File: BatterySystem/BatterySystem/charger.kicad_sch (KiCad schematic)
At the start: 1 part, among them U2 BQ25895RTW

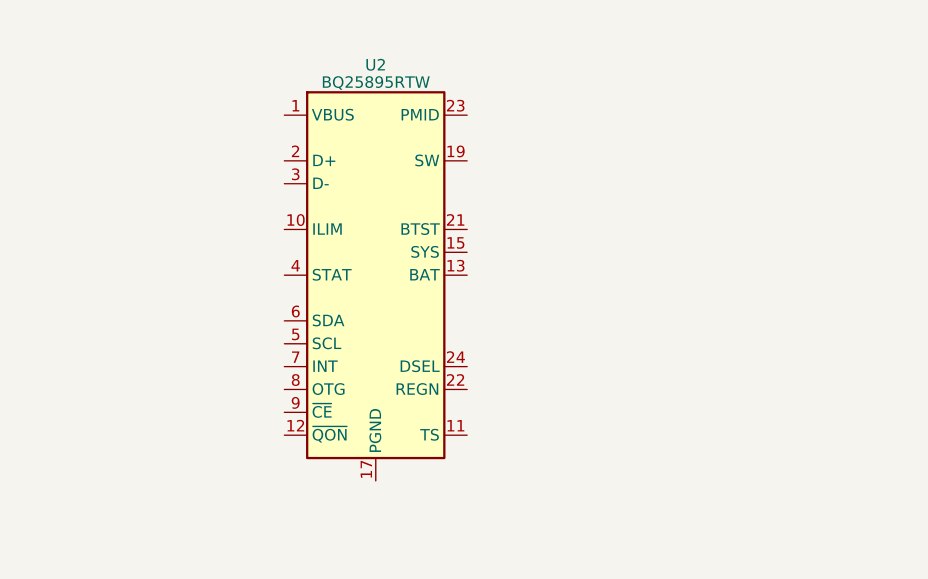
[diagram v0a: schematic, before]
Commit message: Charger circuit gemaakt
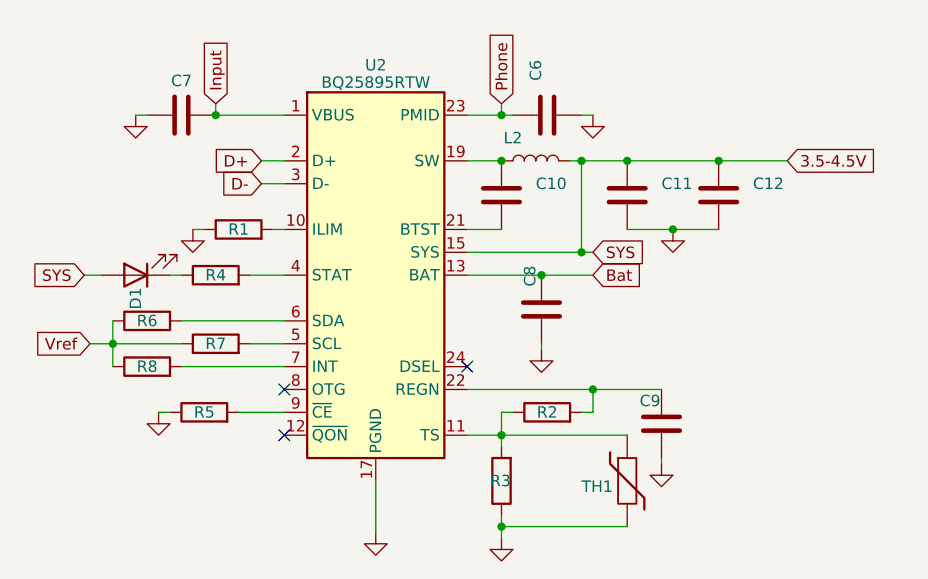
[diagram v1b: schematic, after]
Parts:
- added C10: 47n, symbol Device:C
- added C11, C12, C8: 10u, symbol Device:C
- added C6: 8.2u, symbol Device:C
- added C7: 1u, symbol Device:C
- added C9: 4.7u, symbol Device:C
- added D1: LED, symbol Device:LED
- added L2: 2.2u, symbol Device:L
- added R1: 260, symbol Device:R
- added R2: 5.23k, symbol Device:R
- added R3: 30.1k, symbol Device:R
- added R4: 2.2k, symbol Device:R
- added R5: 4.7k, symbol Device:R
- added R6, R7, R8: 10k, symbol Device:R
- added TH1: Thermistor, symbol Device:Thermistor
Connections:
- net Input: now reaches U2.1 (VBUS)
- net Input: now also C7.1
- net at U2.10 (ILIM): now also R1.2
- net at U2.11 (TS): now also R2.1, R3.2, TH1.1
- net Bat: now reaches U2.13 (BAT), U2.14 (BAT)
- net Bat: now also C8.2
- net 3.5-4.5V: now reaches U2.15 (SYS), U2.16 (SYS)
- net 3.5-4.5V: now also C11.2, C12.2, D1.2 (A), L2.2
- net GND: now reaches U2.17 (PGND), U2.18 (PGND), U2.25 (PGND)
- net GND: now also C11.1, C12.1, C6.2, C7.2, C8.1, C9.1, R1.1, R3.1, R5.1, TH1.2
- net at U2.19 (SW), U2.20 (SW): now also C10.2, L2.1
- net D+: now reaches U2.2 (D+)
- net at U2.21 (BTST): now also C10.1
- net at U2.22 (REGN): now also C9.2, R2.2
- net Phone: now reaches U2.23 (PMID)
- net Phone: now also C6.1
- net D-: now reaches U2.3 (D-)
- net at U2.4 (STAT): now also R4.2
- net at U2.5 (SCL): now also R7.2
- net at U2.6 (SDA): now also R6.2
- net at U2.7 (INT): now also R8.2
- net at U2.9 (~{CE}): now also R5.2
- new net: D1.1 (K), R4.1
- new net Vref: R6.1, R7.1, R8.1
- no-connect marks 0 -> 3
